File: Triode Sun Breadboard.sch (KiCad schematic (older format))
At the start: 20 parts, among them Q1 BC547, Q2 BC547, U1 ECC82

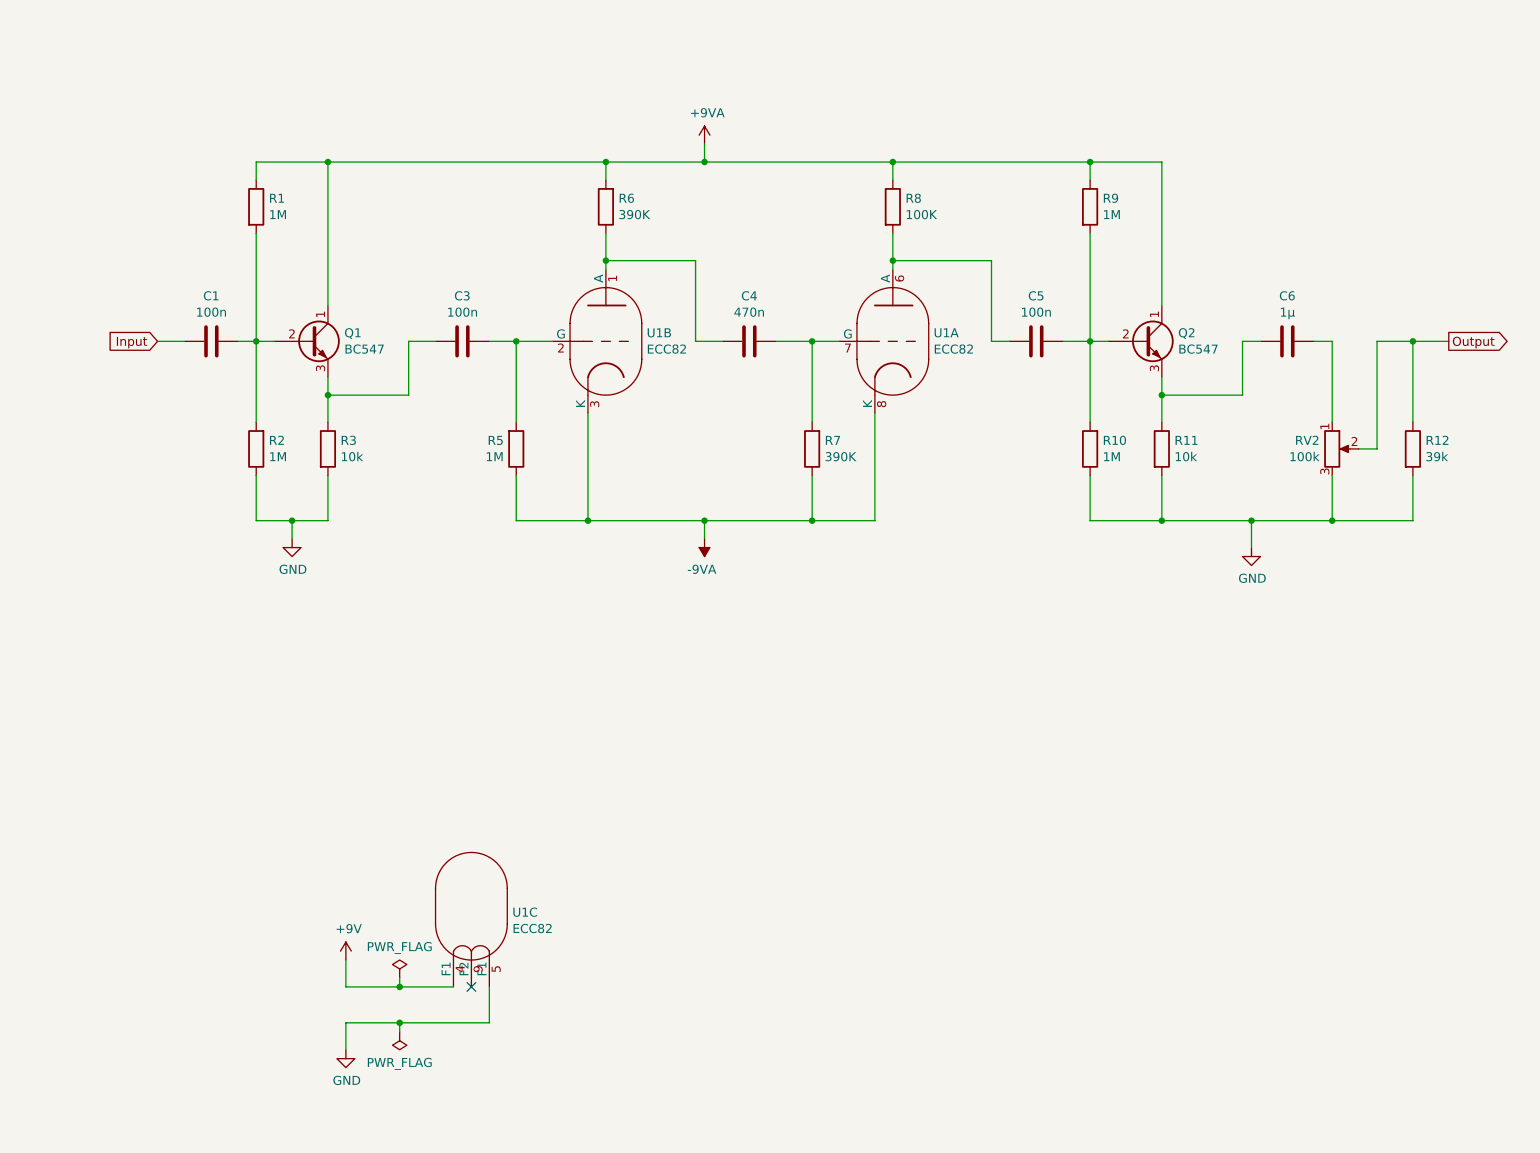
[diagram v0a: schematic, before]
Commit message: Add power supply parts and descriptions
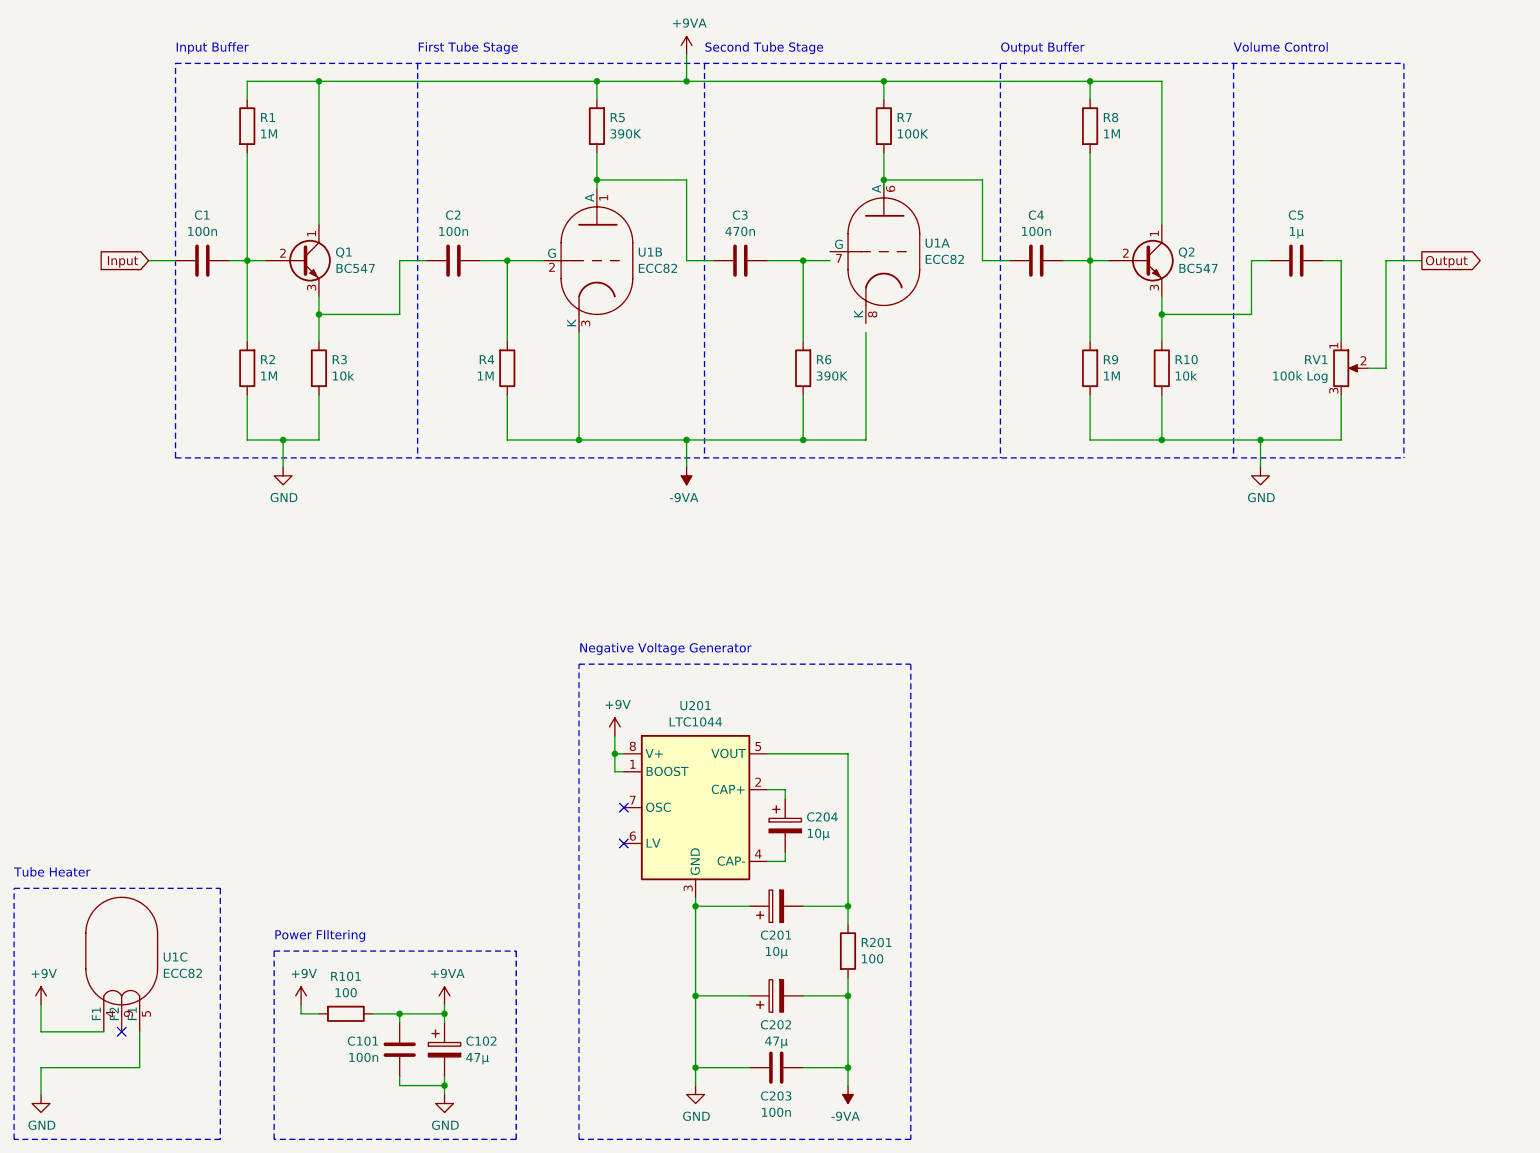
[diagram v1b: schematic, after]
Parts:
- removed C4: 470n, Capacitor_THT:C_Rect_L7.2mm_W3.5mm_P5.00mm_FKS2_FKP2_MKS2_MKP2, symbol Device:C
- removed C6: 1µ, Capacitor_THT:C_Rect_L7.2mm_W4.5mm_P5.00mm_FKS2_FKP2_MKS2_MKP2, symbol Device:C
- removed R12: 39k, Resistor_THT:R_Axial_DIN0207_L6.3mm_D2.5mm_P2.54mm_Vertical, symbol Device:R
- removed R8: 100K, Resistor_THT:R_Axial_DIN0207_L6.3mm_D2.5mm_P2.54mm_Vertical, symbol Device:R
- added C101, C203: 100n, Capacitor_THT:C_Disc_D3.0mm_W1.6mm_P2.50mm, symbol Device:C
- added C102, C202: 47µ, Capacitor_THT:CP_Radial_D5.0mm_P2.50mm, symbol Device:CP
- added C201, C204: 10µ, Capacitor_THT:CP_Radial_D5.0mm_P2.50mm, symbol Device:CP
- added C3: 470n, Capacitor_THT:C_Rect_L7.2mm_W3.5mm_P5.00mm_FKS2_FKP2_MKS2_MKP2, symbol Device:C
- added C5: 1µ, Capacitor_THT:C_Rect_L7.2mm_W4.5mm_P5.00mm_FKS2_FKP2_MKS2_MKP2, symbol Device:C
- added R101: 100, Resistor_THT:R_Axial_DIN0207_L6.3mm_D2.5mm_P2.54mm_Vertical, symbol Device:R
- added R201: 100, Resistor_THT:R_Axial_DIN0207_L6.3mm_D2.5mm_P7.62mm_Horizontal, symbol Device:R
- added R5: 390K, Resistor_THT:R_Axial_DIN0207_L6.3mm_D2.5mm_P2.54mm_Vertical, symbol Device:R
- added U201: LTC1044, Package_DIP:DIP-8_W7.62mm, symbol Regulator_SwitchedCapacitor:LTC1044
- R7: value 390K -> 100K
- RV1: renamed from RV2; value 100k -> 100k Log
- renumbered C3 to C2, C5 to C4, R11 to R10, R5 to R4, R9 to R8, R10 to R9
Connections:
- wire segments 87 -> 114
- no-connect marks 1 -> 3
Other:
- note added: "First Tube Stage"
- note added: "Input Buffer"
- note added: "Negative Voltage Generator"
- note added: "Output Buffer"
- note added: "Power FIltering"
- note added: "Second Tube Stage"
- note added: "Tube Heater"
- note added: "Volume Control"
- moved on the sheet: C2, C4, Q1, Q2, R10, R3, R4, R8, R9, RV1, U1A, U1B
